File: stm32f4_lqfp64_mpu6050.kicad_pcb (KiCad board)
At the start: 4 copper layers, 130 x 100 mm, 156 parts, among them M5 ALIS-CUSTOM-PARTS_POWERPADS, P1 CONN_01X08, P2 CONN_02X08, Q5 BSS138, Q6 CRYSTAL_50X32, U1 STM32F405R, U2 MPU6050, U3 LP2985LV, U4 LP2985LV, U5 W25Q80BV, U6 LM1881, U7 TS5A3160, U8 TS5A3160, X1 CON-JST_SM04B-SRSS-TB, X2 CON-JST_SM04B-SRSS-TB, X4 CON-JST_SM04B-SRSS-TB

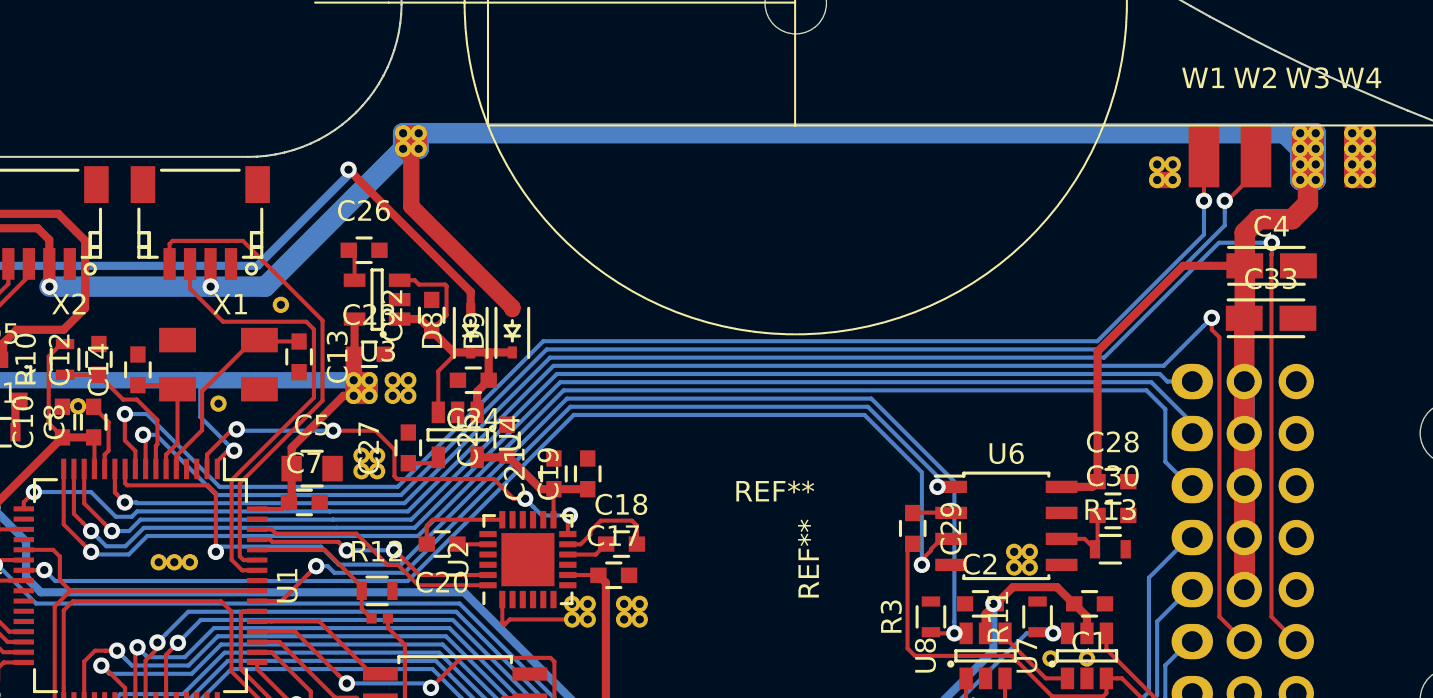
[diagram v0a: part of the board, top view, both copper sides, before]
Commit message: looks better than the rcexplorer naze32
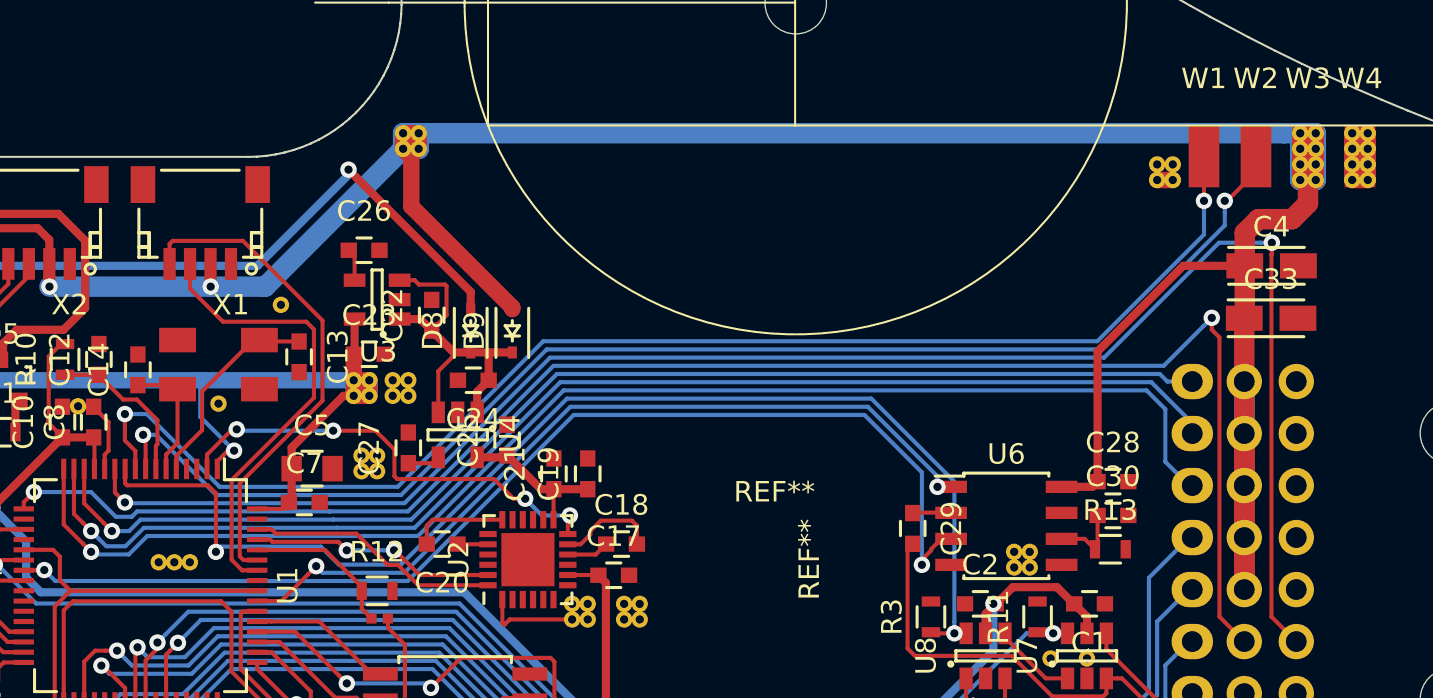
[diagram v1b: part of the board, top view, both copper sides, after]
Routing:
- net VBAT: track 171.4 -> 170.3 mm
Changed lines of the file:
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@@
     (thickness 1.6)
     (drawings 2)
-    (tracks 846)
+    (tracks 843)
     (zones 0)
     (modules 156)
@@
   (segment (start 107.049 98.552) (end 107.049 97.21276) (width 0.4) (layer Top) (net 1))
   (segment (start 107.049 97.21276) (end 107.249 97.01276) (width 0.4) (layer Top) (net 1))
-  (segment (start 169.029998 83.939998) (end 169.022996 83.947) (width 1) (layer Bottom) (net 2))
   (segment (start 169.022996 83.947) (end 126.746 83.947) (width 1) (layer Bottom) (net 2))
   (segment (start 126.746 83.947) (end 126.383999 84.309001) (width 1) (layer Bottom) (net 2))
@@
   (segment (start 170.561 83.947) (end 170.561 86.233) (width 1) (layer Bottom) (net 2))
   (segment (start 170.561 83.947) (end 169.037 83.947) (width 1) (layer Bottom) (net 2))
-  (segment (start 169.037 83.947) (end 169.029998 83.939998) (width 1) (layer Bottom) (net 2))
   (segment (start 167.092 90.424) (end 164.084 90.424) (width 0.4) (layer Top) (net 2))
   (segment (start 164.084 90.424) (end 159.905 94.603) (width 0.4) (layer Top) (net 2))
@@
   (segment (start 170.18 87.376) (end 170.18 85.217) (width 1) (layer Top) (net 2))
   (segment (start 167.755999 88.145001) (end 169.410999 88.145001) (width 1) (layer Top) (net 2))
-  (segment (start 169.799 84.709) (end 169.029998 83.939998) (width 1) (layer Bottom) (net 2))
   (segment (start 167.0685 103.6955) (end 167.0685 106.2355) (width 1) (layer Top) (net 2))
   (segment (start 167.0685 101.1555) (end 167.0685 103.6955) (width 1) (layer Top) (net 2))
@@
   (via (at 116.84 104.394) (size 0.8) (drill 0.4) (layers Top Bottom) (net 42))
   (segment (start 151.82 108.374) (end 151.765 108.319) (width 0.2) (layer Top) (net 42))
+  (segment (start 112.395001 101.981) (end 112.522 101.981) (width 0.2) (layer Bottom) (net 43))
+  (segment (start 112.522 101.981) (end 112.560022 102.019022) (width 0.2) (layer Bottom) (net 43))
+  (segment (start 133.162078 94.907022) (end 160.224378 94.907022) (width 0.2) (layer Bottom) (net 43))
+  (segment (start 112.560022 102.019022) (end 122.231836 102.019022) (width 0.2) (layer Bottom) (net 43))
+  (segment (start 122.233065 102.017793) (end 126.051307 102.017793) (width 0.2) (layer Bottom) (net 43))
   (segment (start 122.231836 102.019022) (end 122.233065 102.017793) (width 0.2) (layer Bottom) (net 43))
-  (segment (start 165.836389 89.295011) (end 167.848421 89.295011) (width 0.2) (layer Bottom) (net 43))
+  (segment (start 167.848421 89.295011) (end 168.414106 89.295011) (width 0.2) (layer Bottom) (net 43))
   (segment (start 126.051307 102.017793) (end 133.162078 94.907022) (width 0.2) (layer Bottom) (net 43))
-  (segment (start 122.233065 102.017793) (end 126.051307 102.017793) (width 0.2) (layer Bottom) (net 43))
-  (segment (start 133.162078 94.907022) (end 160.224378 94.907022) (width 0.2) (layer Bottom) (net 43))
-  (segment (start 112.960686 101.981) (end 112.998708 102.019022) (width 0.2) (layer Bottom) (net 43))
+  (segment (start 165.836389 89.295011) (end 167.848421 89.295011) (width 0.2) (layer Bottom) (net 43))
   (segment (start 160.224378 94.907022) (end 165.836389 89.295011) (width 0.2) (layer Bottom) (net 43))
-  (segment (start 112.998708 102.019022) (end 122.231836 102.019022) (width 0.2) (layer Bottom) (net 43))
-  (segment (start 167.848421 89.295011) (end 168.414106 89.295011) (width 0.2) (layer Bottom) (net 43))
-  (segment (start 112.395001 101.981) (end 112.960686 101.981) (width 0.2) (layer Bottom) (net 43))
   (segment (start 168.414106 89.860696) (end 168.414106 89.295011) (width 0.2) (layer Top) (net 43))
   (segment (start 168.394899 89.879903) (end 168.414106 89.860696) (width 0.2) (layer Top) (net 43))
@@
   (segment (start 121.892 107.795) (end 119.557 107.795) (width 0.2) (layer Top) (net 61))
   (segment (start 119.557 107.795) (end 118.857 107.795) (width 0.2) (layer Top) (net 61))
-  (segment (start 122.627329 105.417867) (end 126.045433 105.417867) (width 0.2) (layer Bottom) (net 62))
-  (segment (start 152.08401 100.70671) (end 152.08401 101.218998) (width 0.2) (layer Bottom) (net 62))
-  (segment (start 134.156212 97.307088) (end 148.684388 97.307088) (width 0.2) (layer Bottom) (net 62))
+  (segment (start 121.737787 105.09401) (end 121.737787 105.100787) (width 0.2) (layer Bottom) (net 62))
+  (segment (start 121.737787 105.100787) (end 122.054867 105.417867) (width 0.2) (layer Bottom) (net 62))
+  (segment (start 122.054867 105.417867) (end 126.045433 105.417867) (width 0.2) (layer Bottom) (net 62))
   (segment (start 148.684388 97.307088) (end 152.08401 100.70671) (width 0.2) (layer Bottom) (net 62))
-  (segment (start 122.303472 105.09401) (end 122.627329 105.417867) (width 0.2) (layer Bottom) (net 62))
-  (segment (start 121.737787 105.09401) (end 122.303472 105.09401) (width 0.2) (layer Bottom) (net 62))
   (segment (start 126.045433 105.417867) (end 134.156212 97.307088) (width 0.2) (layer Bottom) (net 62))
+  (segment (start 134.156212 97.307088) (end 148.684388 97.307088) (width 0.2) (layer Bottom) (net 62))
+  (segment (start 152.08401 100.70671) (end 152.08401 101.218998) (width 0.2) (layer Bottom) (net 62))
   (segment (start 152.649695 101.218998) (end 152.08401 101.218998) (width 0.2) (layer Top) (net 62))
   (segment (start 152.748 101.219) (end 152.747998 101.218998) (width 0.2) (layer Top) (net 62))
